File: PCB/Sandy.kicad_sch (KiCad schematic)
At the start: 163 parts, among them J1 USB_C_Receptacle_USB2.0, J10 Conn_02x02_Top_Bottom, J15 Conn_02x02_Top_Bottom, J2 Conn_01x03, J3 Conn_01x02, J4 Conn_02x03_Odd_Even, J5 Conn_02x02_Top_Bottom, J6 Conn_02x02_Top_Bottom, J7 Conn_02x02_Top_Bottom, J8 Conn_02x02_Top_Bottom, J9 Conn_02x02_Top_Bottom, U1 ATmega32U4-MU, U2 24LC64, Y1 16MHz

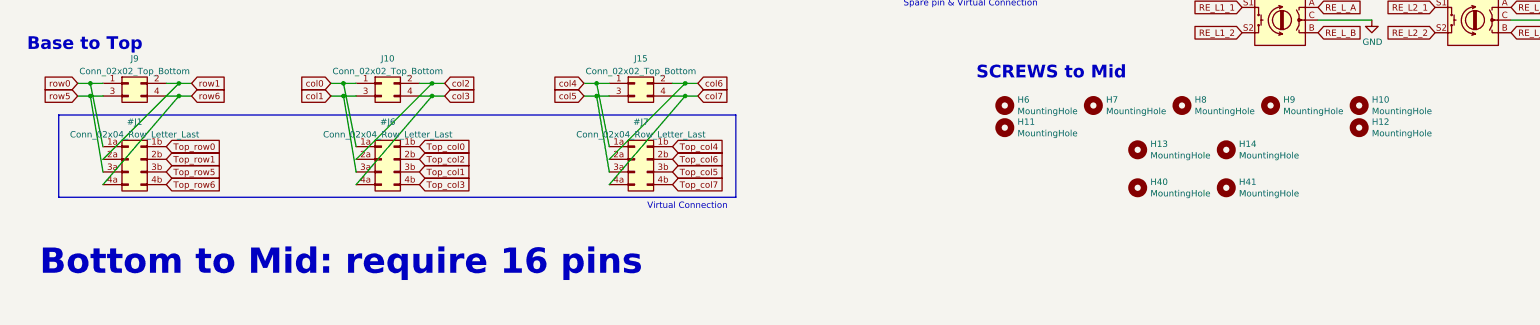
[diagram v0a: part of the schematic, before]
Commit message: 基板外形置き換え
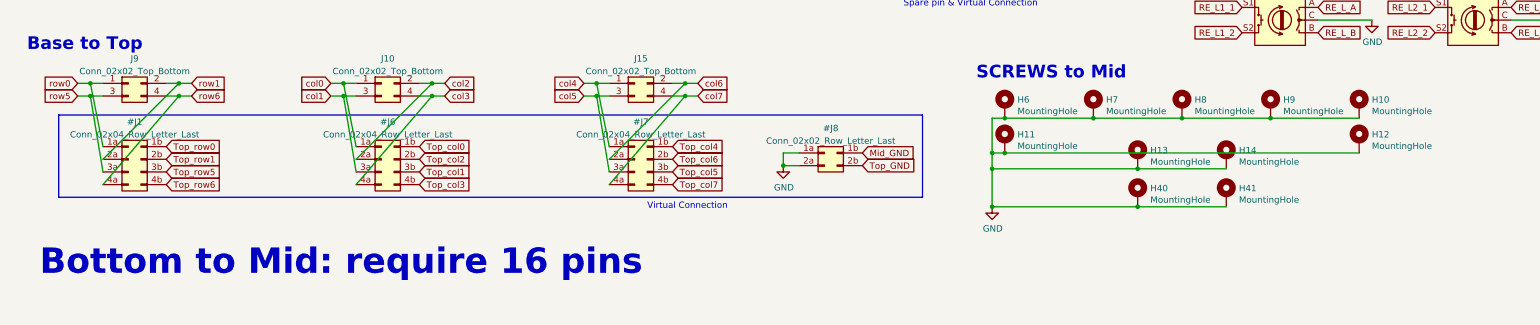
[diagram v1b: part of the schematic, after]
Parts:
- added #J8: Conn_02x02_Row_Letter_Last, symbol Connector_Generic:Conn_02x02_Row_Letter_Last
- H10, H11, H12, H13, H14, H40, H41, H6, H7, H8, H9: footprint MountingHole:MountingHole_2.2mm_M2_No_Cu -> MountingHole:MountingHole_2.2mm_M2_Pad; symbol Mechanical:MountingHole -> Mechanical:MountingHole_Pad
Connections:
- net GND: now also H10.1, H11.1, H12.1, H13.1, H14.1, H40.1, H41.1, H6.1, H7.1, H8.1, H9.1, #J8.1a (Pin_1a), #J8.2a (Pin_2a)
- new net Mid_GND: #J8.1b (Pin_1b)
- new net Top_GND: #J8.2b (Pin_2b)
